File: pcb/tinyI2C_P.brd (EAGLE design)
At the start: 83.2 x 83.2 mm, 274 parts, among them IC1 74LVC1G125DCK, IC10 74LVC1G125DCK, IC11 74LVC1G125DCK, IC12 IC_LDO_MIC5355, IC13 74LVC1G125DCK, IC14 74LVC1G125DCK, IC15 IC_LDO_MIC5355, IC16 74LVC1G125DCK, IC17 74LVC1G125DCK, IC18 IC_LDO_MIC5355, IC19 74LVC1G125DCK, IC2 74LVC1G125DCK, IC20 74LVC1G125DCK, IC21 IC_LDO_MIC5355, IC22 74LVC1G125DCK, IC23 74LVC1G125DCK, IC24 IC_LDO_MIC5355, IC3 IC_LDO_MIC5355, IC4 74LVC1G125DCK, IC5 74LVC1G125DCK, IC6 IC_LDO_MIC5355, IC7 74LVC1G125DCK, IC8 74LVC1G125DCK, IC9 IC_LDO_MIC5355, U1 LPC824M201JHI33, U2 LPC824M201JHI33, U3 LPC824M201JHI33, U4 LPC824M201JHI33, U5 LPC824M201JHI33, U6 LPC824M201JHI33, U7 LPC824M201JHI33, U8 LPC824M201JHI33, X1 TSW-112-02-S-S, X10 TSW-102-02-S-S, X11 TSW-102-02-S-S, X12 TSW-102-02-S-S, X13 TSW-106-02-S-S-RA, X14 TSW-112-02-S-S, X15 TSW-112-02-S-S, X16 TSW-102-02-S-S, X17 TSW-102-02-S-S, X18 TSW-102-02-S-S, X19 TSW-106-02-S-S-RA, X2 TSW-112-02-S-S, X20 TSW-112-02-S-S, X21 TSW-112-02-S-S, X22 TSW-102-02-S-S, X23 TSW-102-02-S-S, X24 TSW-102-02-S-S, X25 TSW-106-02-S-S-RA, X26 TSW-112-02-S-S, X27 TSW-112-02-S-S, X28 TSW-102-02-S-S, X29 TSW-102-02-S-S, X3 TSW-106-02-S-S-RA, X30 TSW-102-02-S-S, X31 TSW-106-02-S-S-RA, X32 TSW-112-02-S-S, X33 TSW-112-02-S-S, X34 TSW-102-02-S-S, X35 TSW-102-02-S-S, X36 TSW-102-02-S-S, X37 TSW-106-02-S-S-RA, X38 TSW-112-02-S-S, X39 TSW-112-02-S-S, X4 TSW-102-02-S-S, X40 TSW-102-02-S-S, X41 TSW-102-02-S-S, X42 TSW-102-02-S-S, X43 TSW-106-02-S-S-RA, X44 TSW-112-02-S-S, X45 TSW-112-02-S-S, X46 TSW-102-02-S-S, X47 TSW-102-02-S-S, X48 TSW-102-02-S-S, X5 TSW-102-02-S-S, X6 TSW-102-02-S-S, X7 TSW-106-02-S-S-RA, X8 TSW-112-02-S-S, X9 TSW-112-02-S-S

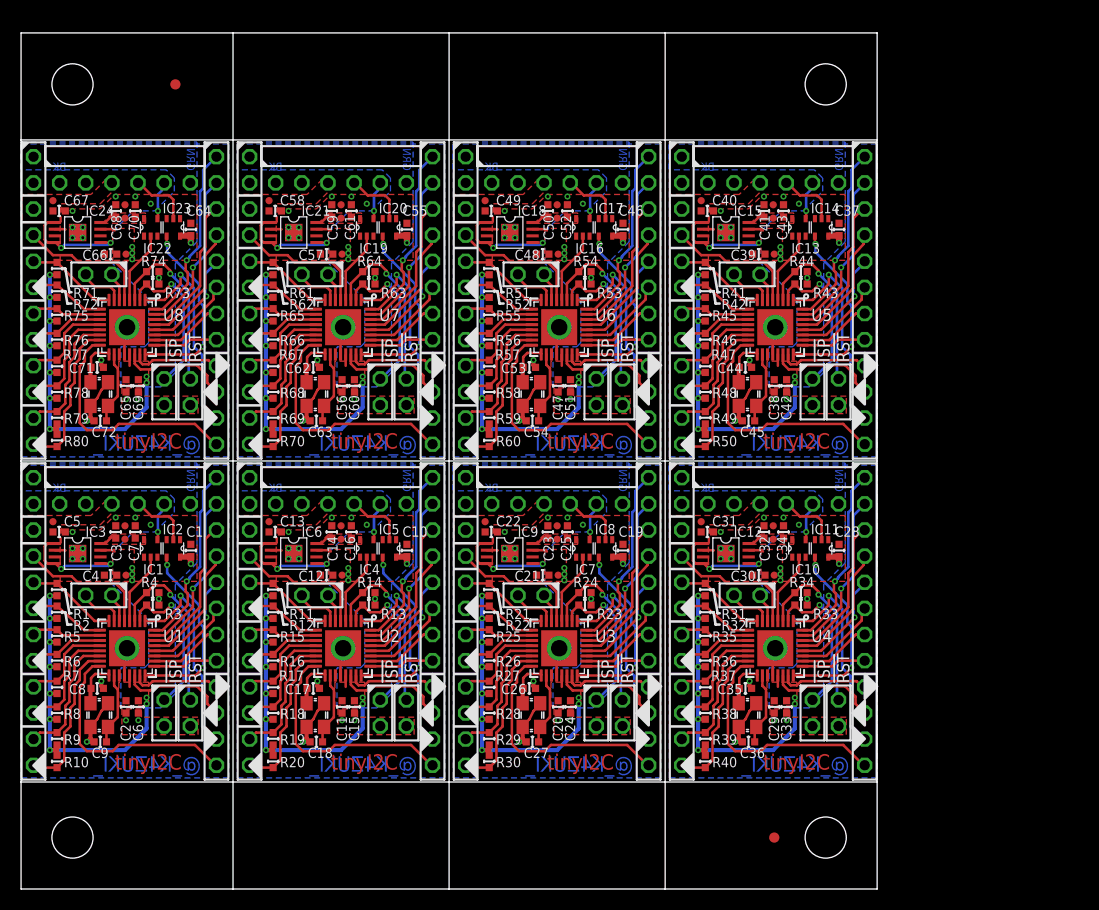
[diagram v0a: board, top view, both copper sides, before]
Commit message: [ PCB ] panelised
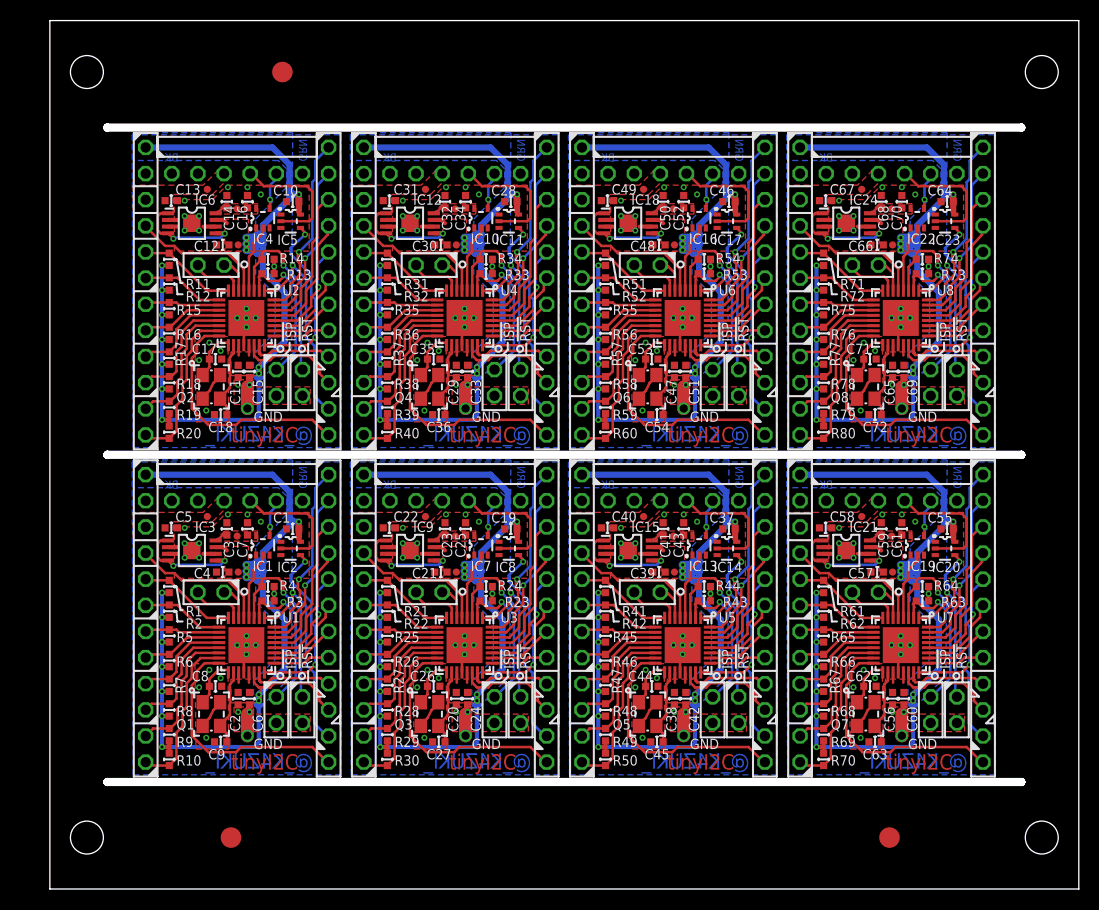
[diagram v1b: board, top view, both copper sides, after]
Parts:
- added I1, I2, I3, I4, I5, I6, I7, I8: ICON_MINLAB_5.2S, mylib:ICON_MINLAB_5.2MM
- added TP35, TP37, TP39, TP40, TP42: TPTP07R, testpad_local:TP07R
- added TP36, TP38, TP41, TP43: TPB1,27, testpad_local:B1,27
- C1, C10, C11, C15, C16, C19, C2, C20, C24, C25, C28, C29, C33, C34, C37, C38, C42, C43, C46, C47, C51, C52, C55, C56, C6, C60, C61, C64, C65, C69, C7, C70: value 1005 -> 0.1u/1005
- C12, C13, C14, C21, C22, C23, C3, C30, C31, C32, C39, C4, C40, C41, C48, C49, C5, C50, C57, C58, C59, C66, C67, C68: value 1005 -> 10u/1005
- C17, C18, C26, C27, C35, C36, C44, C45, C53, C54, C62, C63, C71, C72, C8, C9: value 1005 -> 18p/1005
- IC12, IC15, IC18, IC21, IC24, IC3, IC6, IC9: device mylib:IC_08_0.65_160MIL -> mylib:IC_08_0.65_160MIL_EP
- Q1, Q2, Q3, Q4, Q5, Q6, Q7, Q8: value (none) -> 12MHz
- TP11, TP13, TP16, TP18, TP21, TP23, TP26, TP28, TP3, TP31, TP33, TP7: value TPTP07R -> TPB1,27; device testpad_local:TP07R -> testpad_local:B1,27
- TP4, TP5: value TPTP10R -> TPTP20R; device testpad:TP10R -> testpad_local:TP20R
- TP8: value TPTP07R -> TPTP20R; device testpad_local:TP07R -> testpad_local:TP20R
- moved TP34 77.2 mm to (81.7, 36.2)
- moved C72 75.3 mm to (83.0, 46.1)
- moved U8 75.2 mm to (85.5, 55.5)
- moved C71 75.1 mm to (82.5, 51.5)
- moved IC23 75.0 mm to (89.8, 64.9), turned to 270 degrees
- moved R74 74.8 mm to (87.6, 61.2)
- moved R73 74.8 mm to (87.6, 59.8)
- moved IC24 74.7 mm to (80.2, 64.7)
- moved C65 74.5 mm to (84.7, 50.3)
- moved C67 74.5 mm to (78.2, 66.9)
- moved R79 74.5 mm to (78.0, 46.8)
- moved C66 74.5 mm to (83.2, 62.6)
- moved C70 74.5 mm to (85.6, 66.8)
- moved IC22 74.5 mm to (87.1, 65.2)
- moved R71 74.5 mm to (78.0, 61.2)
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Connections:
- net 1.8V1: now also TP10.TP; no longer TP8.TP
- net 1.8V2: now also TP15.TP; no longer TP12.TP
- net 1.8V3: now also TP20.TP; no longer TP16.TP
- net 1.8V4: now also TP25.TP; no longer TP20.TP
- net 1.8V5: now also TP30.TP; no longer TP24.TP
- net 1.8V6: now also TP35.TP; no longer TP28.TP
- net 1.8V7: now also TP40.TP; no longer TP32.TP
- net 3.3V1: now also TP12.TP; no longer TP10.TP
- net 3.3V2: now also TP17.TP; no longer TP14.TP
- net 3.3V3: now also TP22.TP; no longer TP18.TP
- net 3.3V4: now also TP27.TP; no longer TP22.TP
- net 3.3V5: now also TP32.TP; no longer TP26.TP
- net 3.3V6: now also TP37.TP; no longer TP30.TP
- net 3.3V7: now also TP42.TP; no longer TP34.TP
- net 5V1: now also TP9.TP; no longer TP7.TP
- net 5V2: now also TP14.TP; no longer TP11.TP
- net 5V3: now also TP19.TP; no longer TP15.TP
- net 5V4: now also TP24.TP; no longer TP19.TP
- net 5V5: now also TP29.TP; no longer TP23.TP
- net 5V6: now also TP34.TP; no longer TP27.TP
- net 5V7: now also TP39.TP; no longer TP31.TP
- net GND: now also IC3.3, IC3.6, TP7.TP
- net GND1: now also IC6.3, IC6.6, TP11.TP, TP13.TP; no longer TP9.TP
- net GND2: now also IC9.3, IC9.6, TP16.TP, TP18.TP; no longer TP13.TP
- net GND3: now also IC12.3, IC12.6, TP21.TP, TP23.TP; no longer TP17.TP
- net GND4: now also IC15.3, IC15.6, TP26.TP, TP28.TP; no longer TP21.TP
- net GND5: now also IC18.3, IC18.6, TP31.TP, TP33.TP; no longer TP25.TP
- net GND6: now also IC21.3, IC21.6, TP36.TP, TP38.TP; no longer TP29.TP
- net GND7: now also IC24.3, IC24.6, TP41.TP, TP43.TP; no longer TP33.TP
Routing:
- net 1.8V3: track 39.1 -> 88.4 mm
- net 1.8V: track 39.1 -> 88.4 mm
- net 1.8V2: track 39.1 -> 88.4 mm
- net 1.8V1: track 39.1 -> 88.4 mm
- net 1.8V7: track 39.1 -> 88.4 mm
- net 1.8V4: track 39.1 -> 88.4 mm
- net 1.8V6: track 39.1 -> 88.4 mm
- net 1.8V5: track 39.1 -> 88.4 mm
- net TX->6: track 5.96 -> 12.5 mm
- net TX->7: track 5.96 -> 12.5 mm
- net TX->4: track 5.96 -> 12.5 mm
- net TX->3: track 5.96 -> 12.5 mm
- net TX->5: track 5.96 -> 12.5 mm
- net TX->2: track 5.96 -> 12.5 mm
- net TX->1: track 5.96 -> 12.5 mm
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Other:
- board size 83.2 x 83.2 mm -> 100 x 84.4 mm
- board text added: "GND"
- board text added: "Q1"
- board text added: "V-CUT"
